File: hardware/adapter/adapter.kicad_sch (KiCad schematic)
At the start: 3 parts, among them J1 Conn_01x14_Pin, J2 Conn_01x14_Pin, U1 MAX2121ETI+

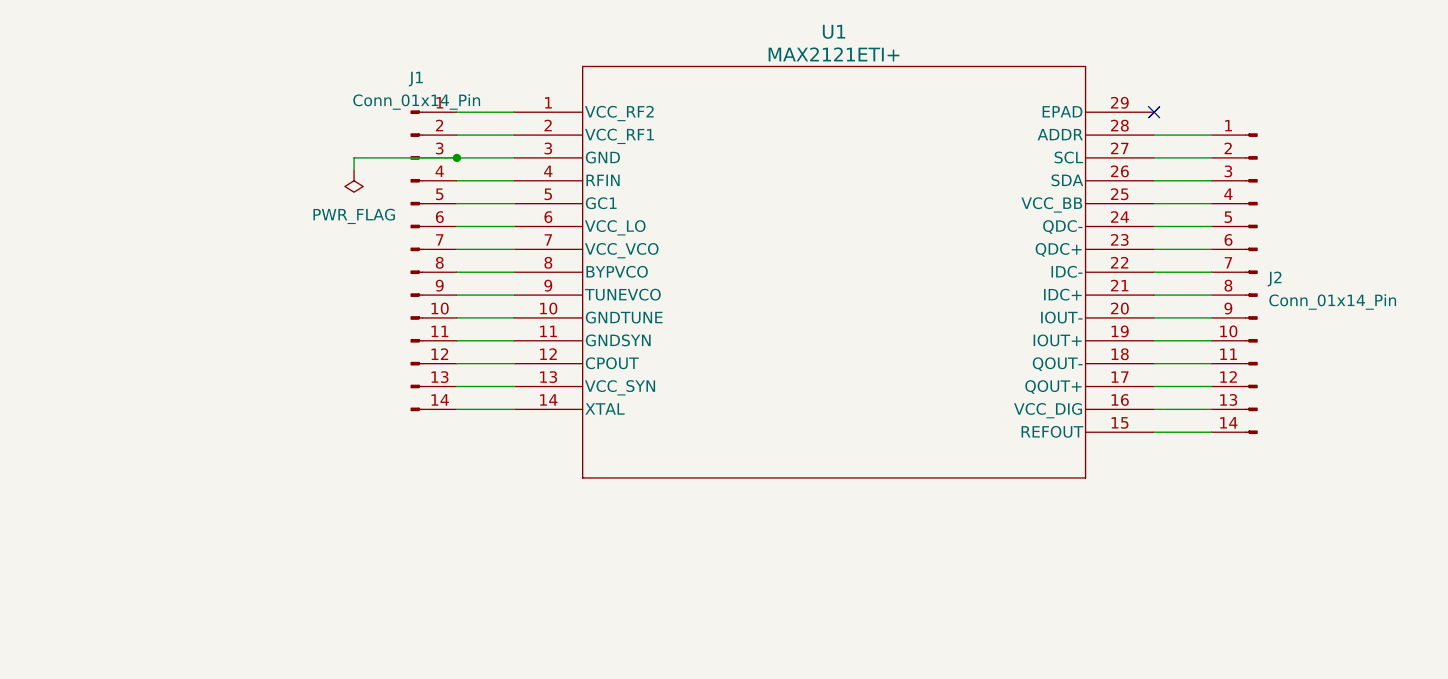
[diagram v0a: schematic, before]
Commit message: fix connector
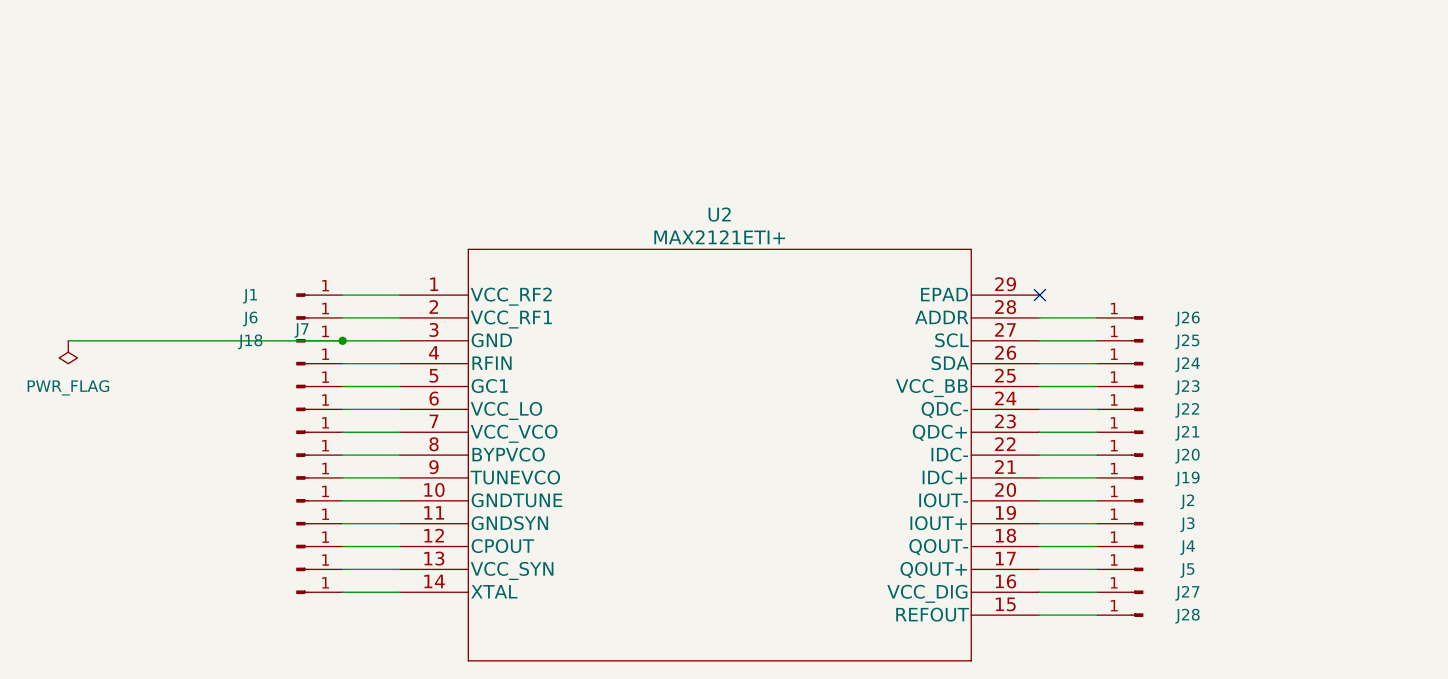
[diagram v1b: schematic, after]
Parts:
- removed J1, J2: Conn_01x14_Pin, Connector_PinHeader_2.54mm:PinHeader_1x14_P2.54mm_Vertical, symbol Connector:Conn_01x14_Pin
- removed U1: MAX2121ETI+, 21-0140L_T2855-3_MXM, symbol MAX2121:MAX2121ETI+
- added J1, J10, J11, J12, J13, J14, J15, J16, J17, J18, J19, J2, J20, J21, J22, J23, J24, J25, J26, J27, J28, J3, J4, J5, J6, J7, J8, J9: Conn_01x01_Pin, Connector_PinHeader_2.54mm:PinHeader_1x01_P2.54mm_Vertical, symbol Connector:Conn_01x01_Pin
- added U2: MAX2121ETI+, footprints:MAX2121ETI&plus_, symbol 2023-05-29_05-01-20:MAX2121ETI+
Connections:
- new net: J27.1 (Pin_1), U2.16 (VCC_DIG)
- new net: J19.1 (Pin_1), U2.21 (IDC+)
- new net: J26.1 (Pin_1), U2.28 (ADDR)
- new net: J3.1 (Pin_1), U2.19 (IOUT+)
- new net: J1.1 (Pin_1), U2.1 (VCC_RF2)
- new net: J13.1 (Pin_1), U2.10 (GNDTUNE)
- new net: J17.1 (Pin_1), U2.11 (GNDSYN)
- new net: J14.1 (Pin_1), U2.12 (CPOUT)
- new net: J15.1 (Pin_1), U2.13 (VCC_SYN)
- new net: J16.1 (Pin_1), U2.14 (XTAL)
- new net: J28.1 (Pin_1), U2.15 (REFOUT)
- new net: J5.1 (Pin_1), U2.17 (QOUT+)
- new net: J4.1 (Pin_1), U2.18 (QOUT-)
- new net: J6.1 (Pin_1), U2.2 (VCC_RF1)
- new net: J2.1 (Pin_1), U2.20 (IOUT-)
- new net: J20.1 (Pin_1), U2.22 (IDC-)
- new net: J21.1 (Pin_1), U2.23 (QDC+)
- new net: J22.1 (Pin_1), U2.24 (QDC-)
- new net: J23.1 (Pin_1), U2.25 (VCC_BB)
- new net: J24.1 (Pin_1), U2.26 (SDA)
- new net: J25.1 (Pin_1), U2.27 (SCL)
- new net: J18.1 (Pin_1), U2.3 (GND)
- new net: J7.1 (Pin_1), U2.4 (RFIN)
- new net: J8.1 (Pin_1), U2.5 (GC1)
- new net: J9.1 (Pin_1), U2.6 (VCC_LO)
- new net: J10.1 (Pin_1), U2.7 (VCC_VCO)
- new net: J11.1 (Pin_1), U2.8 (BYPVCO)
- new net: J12.1 (Pin_1), U2.9 (TUNEVCO)
